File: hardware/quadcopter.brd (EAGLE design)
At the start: 126.2 x 126.2 mm, 85 parts, among them J1 AVR_SPI_PRG_6-SMD, J2 HEADER-4POS-0.1IN-FEMALE-SMD-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, J3 HEADER-10POSTH-254X10, J4 HEADER-4POS-0.1IN-FEMALE-SMD-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, M1 MOTOR_PADS_GND-MOLEX-SMD, M2 MOTOR_PADS_GND-MOLEX-SMD, M3 MOTOR_PADS_GND-MOLEX-SMD, M4 MOTOR_PADS_GND-MOLEX-SMD, Q1 MOSFET-SI2302CDS-T1-E3CT-ND, Q2 MOSFET-SI2302CDS-T1-E3CT-ND, Q3 MOSFET-SI2302CDS-T1-E3CT-ND, Q4 MOSFET-SI2302CDS-T1-E3CT-ND, Q5 MOSFET-SI2302CDS-T1-E3CT-ND, Q6 MOSFET-SI2302CDS-T1-E3CT-ND, Q7 MOSFET-SI2302CDS-T1-E3CT-ND, Q8 MOSFET-SI2302CDS-T1-E3CT-ND, Q9 MOSFET-SI2302CDS-T1-E3CT-ND, SW1 PUSHBUTTON_SMD-VERTICAL-1, U1 ATMEGA128RFA1, U2 LSM-IMU-497-18367-1-NDIMU, Y1 CRYSTAL5X3

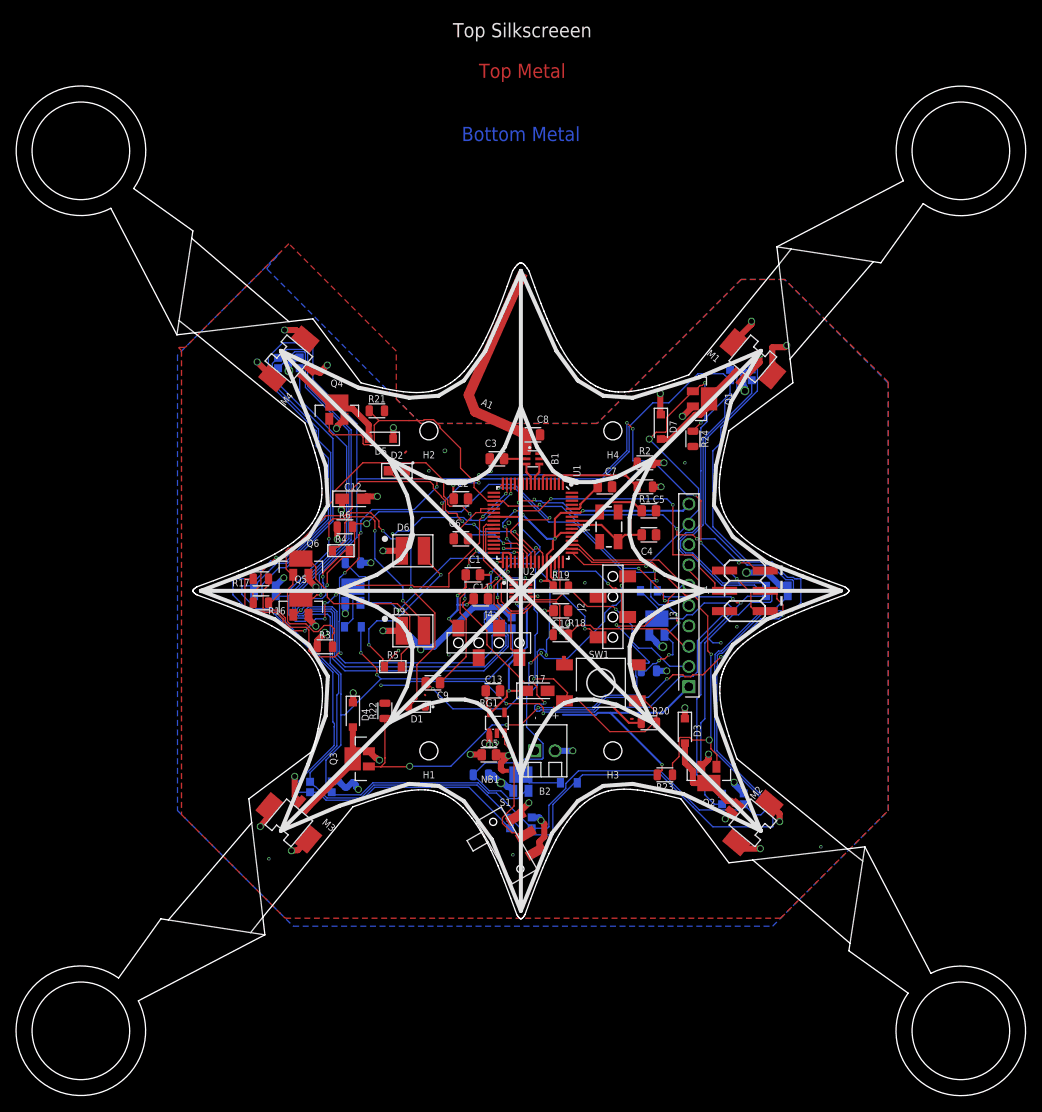
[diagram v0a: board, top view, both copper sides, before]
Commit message: tapeout
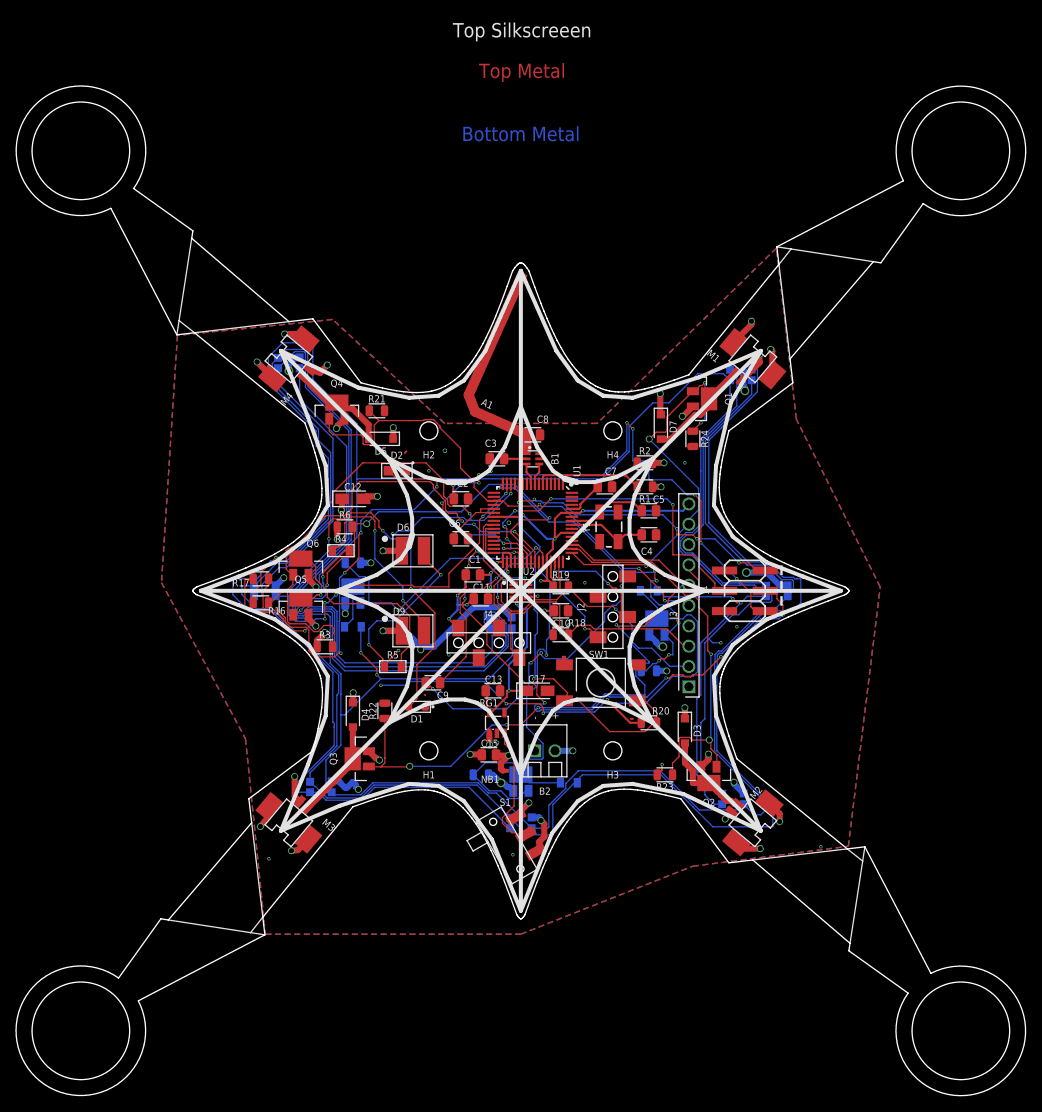
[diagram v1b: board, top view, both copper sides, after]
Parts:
- moved U$1 18.3 mm to (-0.13, -20.7)
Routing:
- net GND: track 48.8 -> 22.5 mm
- net N$19: track 68.5 -> 60.3 mm
- net BAT_GND: track 61.0 -> 58.7 mm
- net PWM3: track 83.7 -> 85.2 mm
- net MISO: track 78.3 -> 79.7 mm

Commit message: tapeout quick check update
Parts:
- renumbered U$1 to LG1
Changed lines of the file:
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@@
 <element name="DECO1" library="quadparts_prebuilt_2022" package="LAYER_LABELS" value="DECORATION-LAYER-LABELS" x="0" y="74" smashed="yes">
 </element>
-<element name="U$1" library="custom_" library_urn="urn:adsk.wipprod:fs.file:vf.FjMADskDQ2Se9fX1PD5xcw" package="VORTEX-LOGO" value="" x="-0.128" y="-20.661" smashed="yes" rot="MR0">
+<element name="LG1" library="custom_" library_urn="urn:adsk.wipprod:fs.file:vf.FjMADskDQ2Se9fX1PD5xcw" package="VORTEX-LOGO" value="" x="-0.128" y="-20.661" smashed="yes" rot="MR0">
 </element>
 <element name="J1" library="quadparts_prebuilt_2022" package="2X3-SMD" value="AVR_SPI_PRG_6-SMD" x="28" y="0" smashed="yes" rot="R90">
